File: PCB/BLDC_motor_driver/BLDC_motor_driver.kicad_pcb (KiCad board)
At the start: 2 copper layers, 11 parts, among them Q2 CSD18534Q5A, Q3 CSD18540Q5B, Q4 CSD18533Q5A, U1 INA240A1D, U2 AS5048A, U3 IR2104, U4 UCC27714D, U5 SN65HVD230, U6 STM32F405RGTx, U7 STM32F303K8Tx, U8 INA240A1D

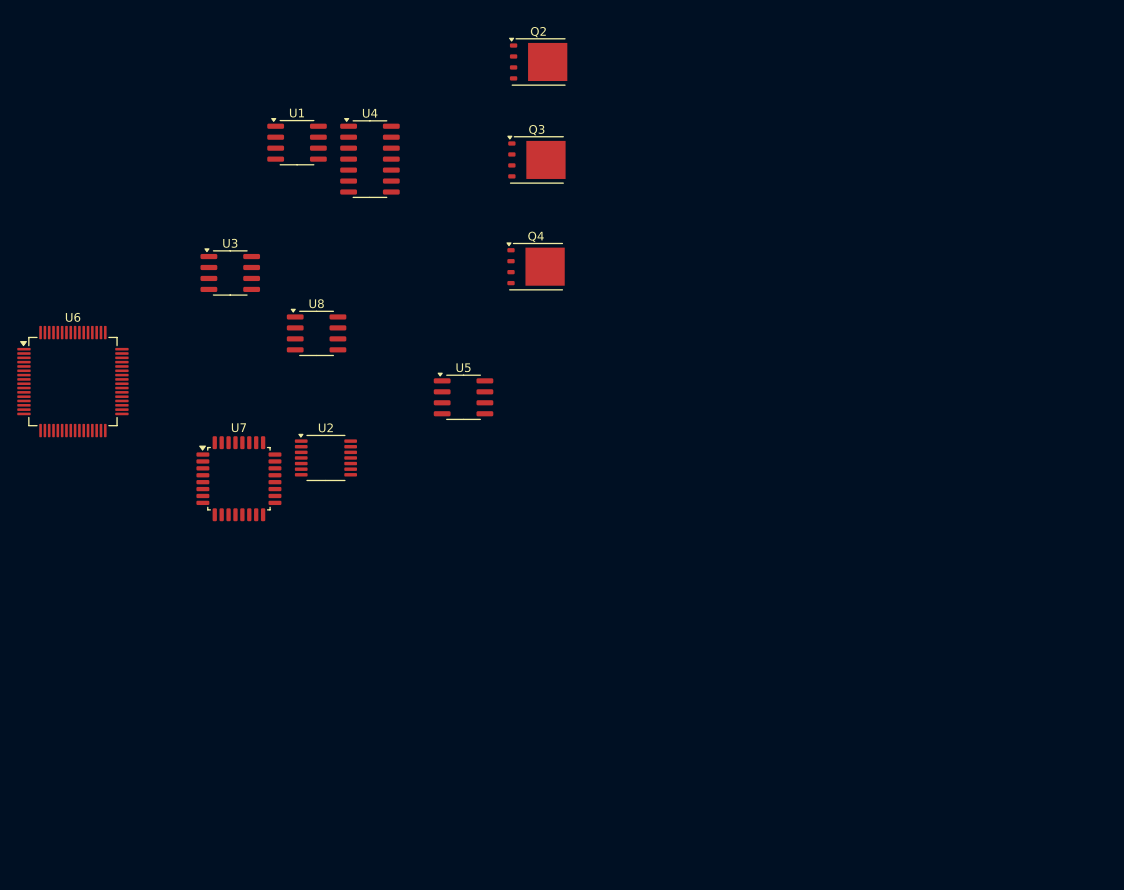
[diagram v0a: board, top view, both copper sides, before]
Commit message: pcb progress
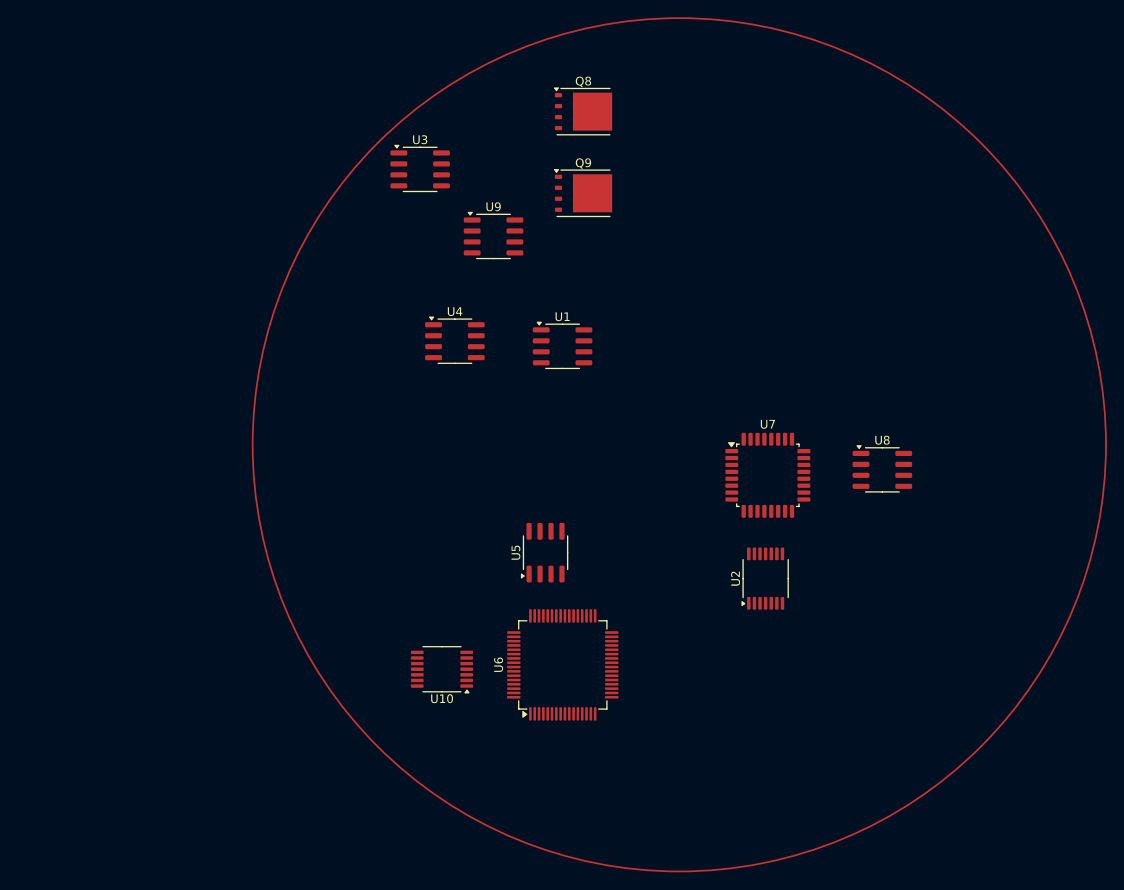
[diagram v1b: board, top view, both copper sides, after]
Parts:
- removed Q2: CSD18534Q5A, Package_TO_SOT_SMD:TDSON-8-1
- removed Q3: CSD18540Q5B, Package_TO_SOT_SMD:TDSON-8-1
- removed Q4: CSD18533Q5A, Package_TO_SOT_SMD:TDSON-8-1
- added Q8: CSD18533Q5A, Package_TO_SOT_SMD:TDSON-8-1, F.Cu at (115.9, 44.4)
- added Q9: CSD18533Q5A, Package_TO_SOT_SMD:TDSON-8-1, F.Cu at (115.9, 53.9)
- added U10: AS5048A, Package_SO:TSSOP-14_4.4x5mm_P0.65mm, F.Cu at (99.5, 109.0)
- added U9: INA240A1D, Package_SO:SOIC-8_3.9x4.9mm_P1.27mm, F.Cu at (105.5, 58.9)
- U1: value INA240A1D -> INA240A2D
- U4: value UCC27714D -> INA240A3D; footprint Package_SO:SOIC-14_3.9x8.7mm_P1.27mm -> Package_SO:SOIC-8_3.9x4.9mm_P1.27mm
- U8: value INA240A1D -> SN65HVD230
- moved U8 67.4 mm to (150.5, 85.9)
- moved U6 65.6 mm to (113.5, 108.5), turned to 90 degrees
- moved U7 61.3 mm to (137.3, 86.5)
- moved U2 52.8 mm to (137.0, 98.5), turned to 90 degrees
- moved U1 38.8 mm to (113.5, 71.6)
- moved U3 25.1 mm to (97.0, 51.1)
- moved U4 23.3 mm to (101.0, 71.0)
- moved U5 20.4 mm to (111.5, 95.5), turned to 90 degrees
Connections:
- U2 pad 1: unconnected-(U2-~{CSn}-Pad1) -> STM1_SPI1_CS
- U2 pad 2: unconnected-(U2-CLK-Pad2) -> STM1_SPI1_SCK
- U2 pad 3: unconnected-(U2-MISO-Pad3) -> STM1_SPI1_MISO
- U2 pad 4: unconnected-(U2-MOSI-Pad4) -> STM1_SPI1_MOSI
- U3 pad 1: unconnected-(U3-VCC-Pad1) -> /BLDC driver phase A/PWR_12V
- U3 pad 2: unconnected-(U3-IN-Pad2) -> /BLDC driver phase A/PWM_IN_A
- U3 pad 3: unconnected-(U3-~{SD}-Pad3) -> /BLDC driver phase A/SD_A
- U3 pad 4: unconnected-(U3-COM-Pad4) -> Net-(U3-COM)
- U3 pad 5: unconnected-(U3-LO-Pad5) -> Net-(U3-LO)
- U3 pad 6: unconnected-(U3-VS-Pad6) -> /BLDC driver phase A/PHASE A
- U3 pad 7: unconnected-(U3-HO-Pad7) -> Net-(U3-HO)
- U3 pad 8: unconnected-(U3-VB-Pad8) -> Net-(U3-VB)
- U4 pad 2: unconnected-(U4-LI-Pad2) -> Net-(U4-GND-Pad2)
- U4 pad 4: unconnected-(U4-EN/NC-Pad4) -> Net-(U4-GND-Pad2)
- U5 pad 1: unconnected-(U5-D-Pad1) -> STM2_CAN_TX
- U5 pad 4: unconnected-(U5-R-Pad4) -> STM2_CAN_RX
- U6 pad 21: unconnected-(U6-PA5-Pad21) -> STM2_SPI1_SCK
- U6 pad 22: unconnected-(U6-PA6-Pad22) -> STM2_SPI1_MISO
- U6 pad 23: unconnected-(U6-PA7-Pad23) -> STM2_SPI1_MOSI
- U6 pad 24: unconnected-(U6-PC4-Pad24) -> STM2_SPI1_CS
- U6 pad 44: unconnected-(U6-PA11-Pad44) -> STM2_CAN_RX
- U6 pad 45: unconnected-(U6-PA12-Pad45) -> STM2_CAN_TX
- U7 pad 11: unconnected-(U7-PA5-Pad11) -> STM1_SPI1_SCK
- U7 pad 12: unconnected-(U7-PA6-Pad12) -> STM1_SPI1_MISO
- U7 pad 13: unconnected-(U7-PA7-Pad13) -> STM1_SPI1_MOSI
- U7 pad 18: unconnected-(U7-PA8-Pad18) -> STM1_SPI1_CS
- U7 pad 21: unconnected-(U7-PA11-Pad21) -> STM1_CAN_RX
- U7 pad 22: unconnected-(U7-PA12-Pad22) -> STM1_CAN_TX
- U8 pad 1: unconnected-(U8---Pad1) -> STM1_CAN_TX
- U8 pad 2: Net-(U8-GND-Pad2) -> unconnected-(U8-GND-Pad2)
- U8 pad 4: Net-(U8-GND-Pad2) -> STM1_CAN_RX
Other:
- copper layers 2 -> 4
